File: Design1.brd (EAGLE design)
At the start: 45.1 x 50.2 mm, 30 parts, among them U1 ATMEGA328P-AU

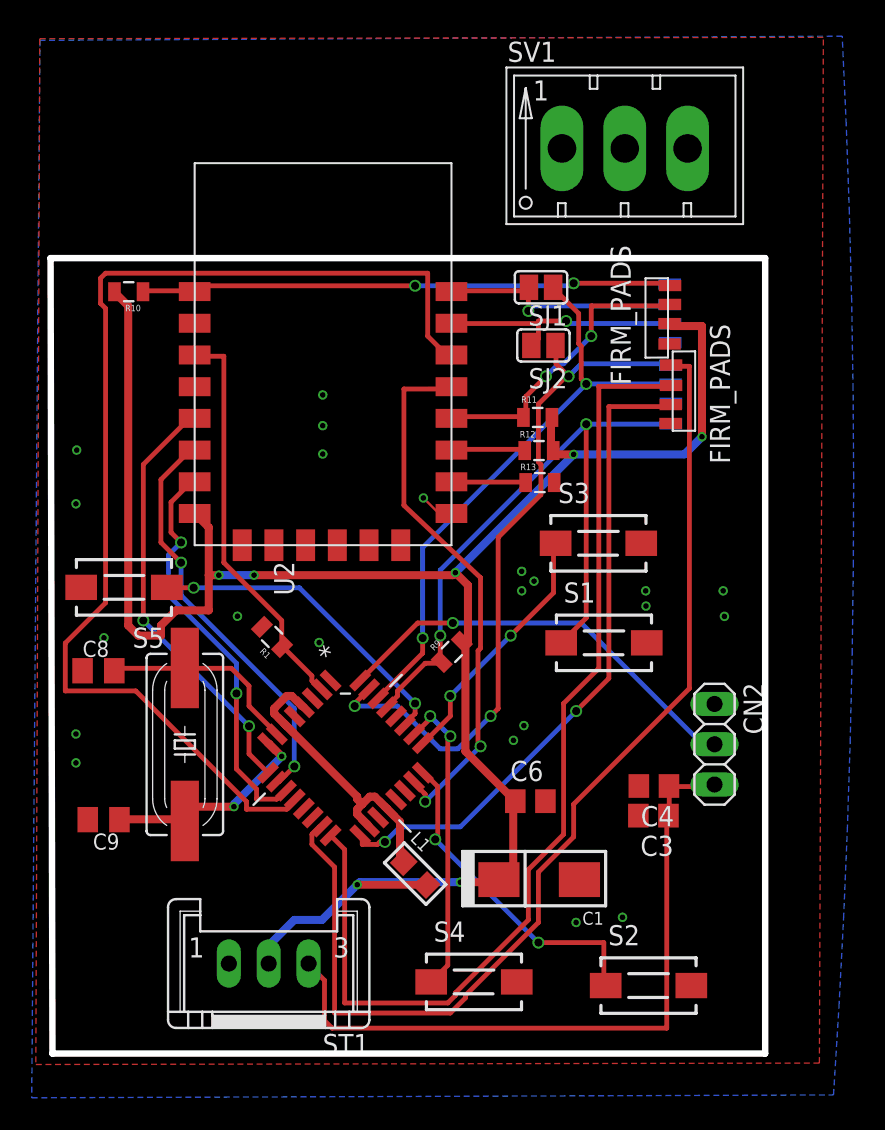
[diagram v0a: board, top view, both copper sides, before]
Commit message: v 0.5 good
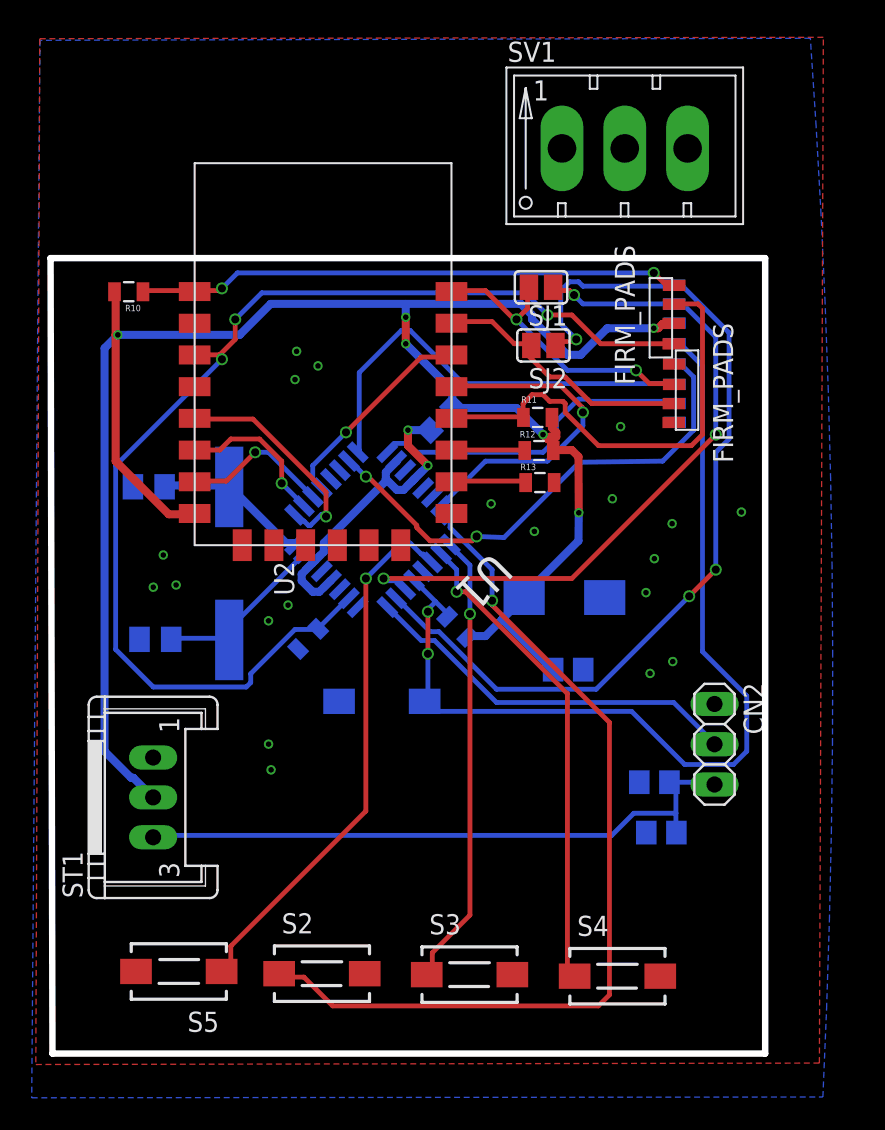
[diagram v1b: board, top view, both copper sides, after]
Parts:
- removed MCU_FIRM1, MCU_FIRM2, MCU_FIRM3, U$3: FIRM_PADSSMD_FIRM_PADS, firm_pads:FIRM_PADS
- added CON1: AT1, firm_pads:FIRM_PADS
- added CON2: AT2, firm_pads:FIRM_PADS
- added CON3: ESP1, firm_pads:FIRM_PADS
- added CON4: ESP2, firm_pads:FIRM_PADS
- S1: value DTSM-3 -> RESET_A
- S2: value DTSM-3 -> UPDATE
- S3: value DTSM-3 -> CONFIG
- S4: value DTSM-3 -> RESET
- S5: value DTSM-3 -> TEST
- moved L1 28.7 mm to (27.5, 43.0), flipped to the bottom, turned to 135 degrees
- moved S3 28.4 mm to (29.3, 7.98)
- moved S5 24.5 mm to (11.0, 8.18)
- moved C9 21.2 mm to (9.08, 38.8), flipped to the bottom, turned to 0 degrees
- moved S2 20.6 mm to (20.0, 8.04)
- moved C1 17.9 mm to (35.3, 31.8), flipped to the bottom, turned to 0 degrees
- moved ST1 16.3 mm to (6.81, 19.2), turned to 90 degrees
- moved U1 14.5 mm to (23.2, 36.0), flipped to the bottom, turned to 135 degrees
- moved S1 14.5 mm to (23.8, 25.2), flipped to the bottom
- moved OSC1 11.8 mm to (14.2, 33.9), flipped to the bottom, turned to 90 degrees
- moved S4 9.06 mm to (38.6, 7.88)
- moved C6 8.63 mm to (35.5, 27.2), flipped to the bottom, turned to 180 degrees
- moved C8 4.10 mm to (9.49, 29.1), flipped to the bottom, turned to 180 degrees
- moved R1 2.28 mm to (19.1, 29.2), flipped to the bottom, turned to 315 degrees
- moved R9 1.62 mm to (28.5, 29.9), flipped to the bottom, turned to 225 degrees
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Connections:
- net N$11 renamed AT_VCC
- removed net N$1: MCU_FIRM3.1
- removed net N$17: MCU_FIRM1.4
- net +3V3: now also CON3.2; no longer MCU_FIRM3.2
- net CH_PD: now also CON3.1
- net GND: now also CON1.4, CON4.4; no longer MCU_FIRM2.2, U$3.4
- net GPIO0: now also CON3.3; no longer MCU_FIRM3.3
- net MISO: now also CON1.2; no longer MCU_FIRM1.2
- net MOSI: now also CON1.1; no longer MCU_FIRM1.1
- net N$4: now also CON4.1; no longer U$3.1
- net RST_A: now also CON2.1; no longer MCU_FIRM2.1
- net RST_E: now also CON3.4; no longer MCU_FIRM3.4
- net RX: now also CON2.4; no longer MCU_FIRM2.4
- net RXD_FIRM: now also CON4.2; no longer U$3.2
- net SCK: now also CON1.3; no longer MCU_FIRM1.3
- net TX: now also CON2.3; no longer MCU_FIRM2.3
- net TXD_FIRM: now also CON4.3; no longer U$3.3
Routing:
- net ESP_ACK: track 72.1 -> 13.3 mm, vias 0 -> 1
- net CH_PD: track 25.5 -> 73.7 mm, vias 0 -> 3
- net MISO: track 64.9 -> 27.4 mm
- net MOSI: track 68.2 -> 31.7 mm, vias 0 -> 2
- net BTN_UPDATE: track 20.8 -> 56.4 mm, vias 2 -> 1
- net SCK: track 41.6 -> 20.8 mm, vias 2 -> 0
- net RST_A: track 43.5 -> 60.1 mm
- net ESP_UPDATE: track 25.9 -> 9.41 mm, vias 2 -> 1
- net ESP_CONFIG: track 26.0 -> 9.77 mm, vias 2 -> 1
- net BTN_TEST: track 20.3 -> 34.2 mm, vias 2 -> 1
- net RX: track 44.8 -> 58.2 mm
- net ESP_OK: track 34.3 -> 21.1 mm, vias 2 -> 1
- net ESP_MOTION: track 27.1 -> 14.3 mm, vias 2 -> 1
- net BTN_CONFIG: track 16.1 -> 28.8 mm, vias 2 -> 1
- net BTN_RESET: track 19.4 -> 30.5 mm, vias 2 -> 1
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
